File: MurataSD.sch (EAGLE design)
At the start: 5 parts, among them U1 IC_BLE_LBCA2HNZYZ-711, U2 BOARD_MMC, X1 TSW-103-02-S-S

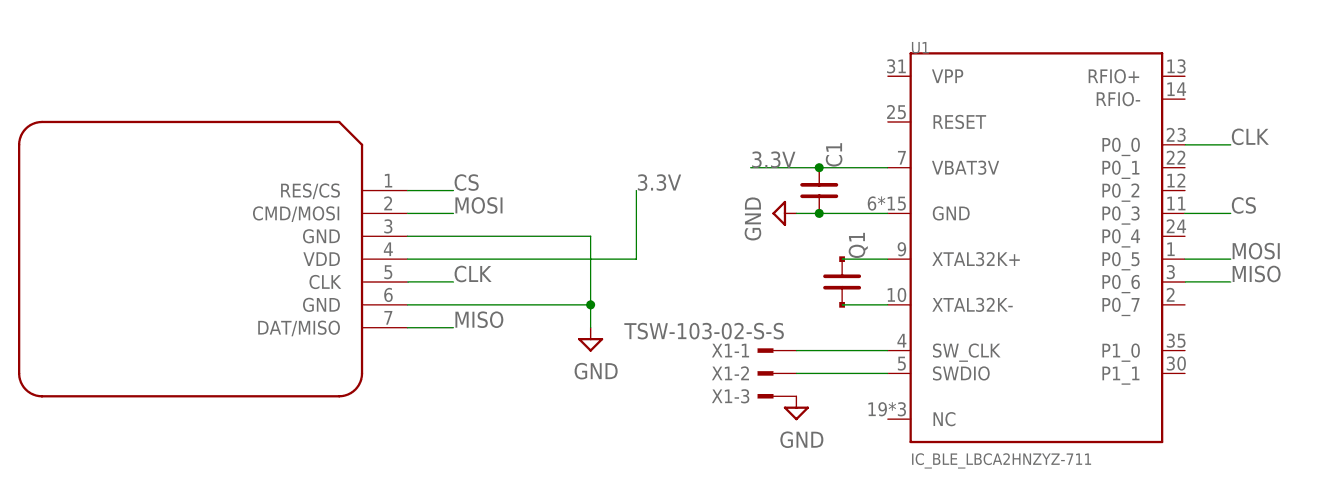
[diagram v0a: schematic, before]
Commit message: [ SD ] update library
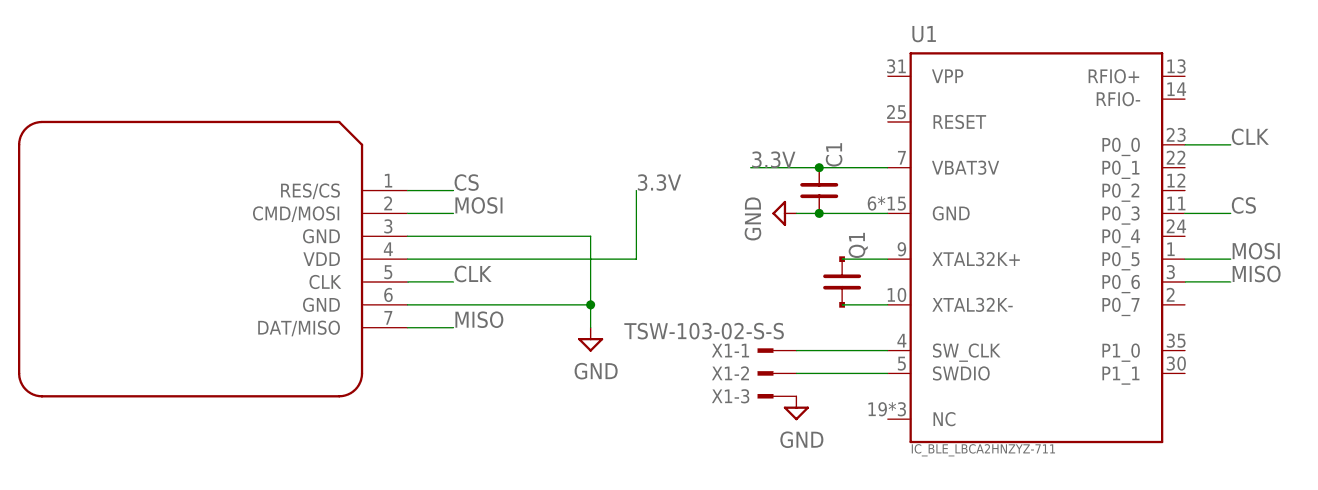
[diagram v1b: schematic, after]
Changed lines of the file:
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@@
 <layers>
 <layer number="1" name="Top" color="4" fill="1" visible="no" active="no"/>
+<layer number="2" name="Route2" color="1" fill="3" visible="no" active="no"/>
+<layer number="3" name="Route3" color="4" fill="3" visible="no" active="no"/>
+<layer number="14" name="Route14" color="1" fill="6" visible="no" active="no"/>
+<layer number="15" name="Route15" color="4" fill="6" visible="no" active="no"/>
 <layer number="16" name="Bottom" color="1" fill="1" visible="no" active="no"/>
 <layer number="17" name="Pads" color="2" fill="1" visible="no" active="no"/>
@@
 <layer number="132" name="bAdjust" color="7" fill="1" visible="no" active="yes"/>
 <layer number="144" name="Drill_legend" color="7" fill="1" visible="yes" active="yes"/>
+<layer number="145" name="DrillLegend_01-16" color="2" fill="9" visible="no" active="yes"/>
+<layer number="146" name="DrillLegend_01-20" color="3" fill="9" visible="no" active="yes"/>
 <layer number="151" name="HeatSink" color="7" fill="1" visible="yes" active="yes"/>
 <layer number="152" name="_bDocu" color="7" fill="1" visible="yes" active="yes"/>
